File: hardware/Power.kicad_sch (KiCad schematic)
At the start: 8 parts, among them U201 TPS62172DSGR

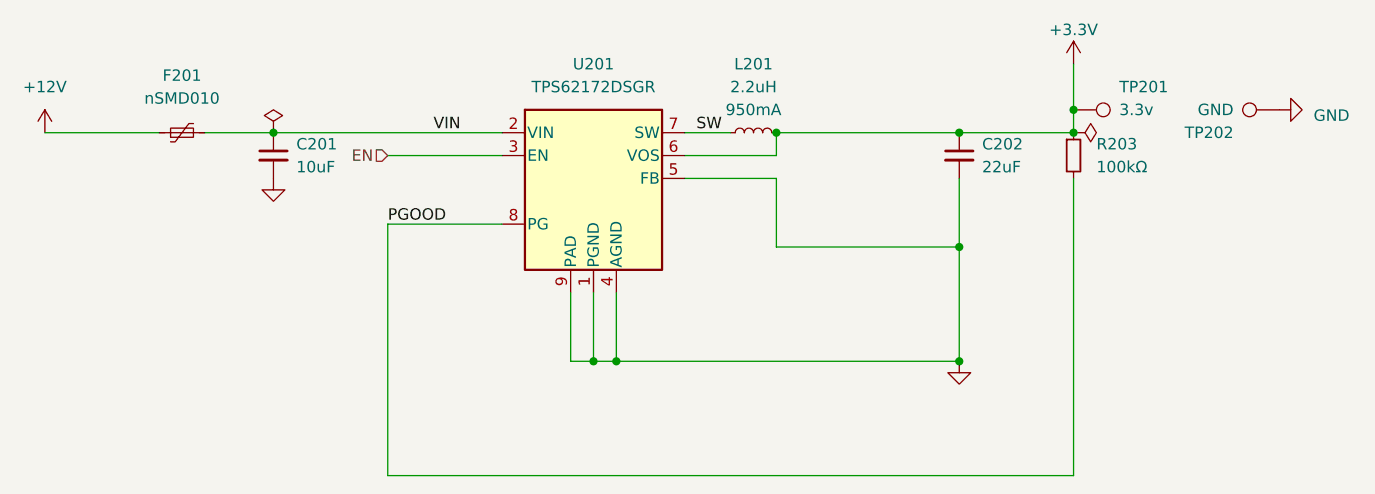
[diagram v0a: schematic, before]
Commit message: Almost ready for fab
Signed-off-by: Connor Rigby <connorr@hey.com>
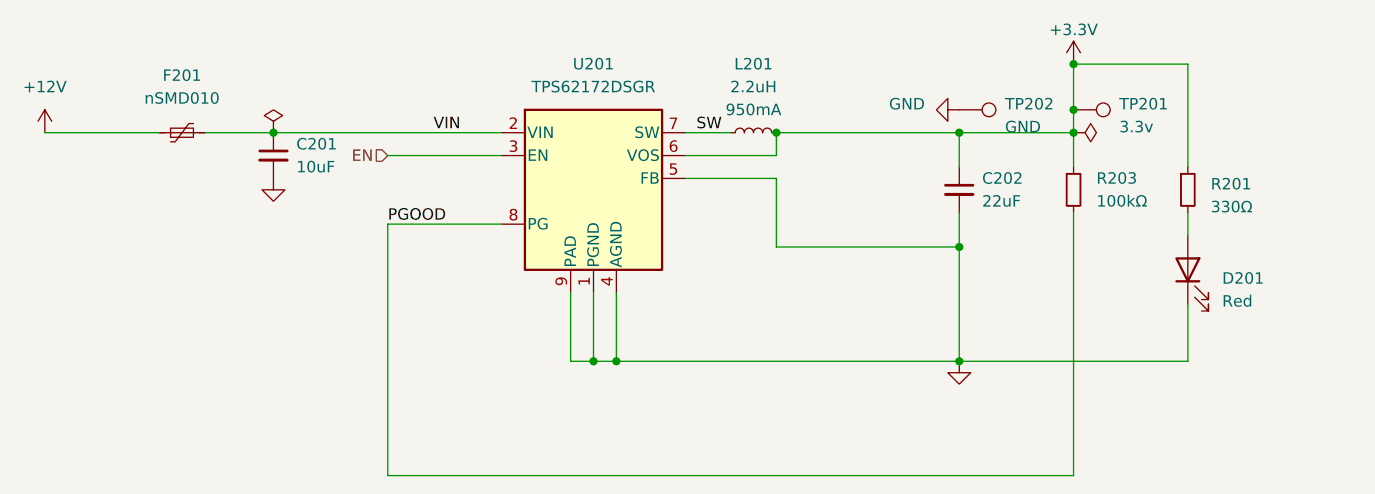
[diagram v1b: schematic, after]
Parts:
- added D201: LED_0603_RED, LED_SMD:LED_0603_1608Metric, symbol LCSC_LED:LED_0603_RED
- added R201: R_0603_330, Resistor_SMD:R_0603_1608Metric, symbol LCSC_Resistor:R_0603_330
- TP201, TP202: now left out of the parts list
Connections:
- net +3.3V: now also R201.1
- net GND: now also D201.1 (K)
- new net: D201.2 (A), R201.2
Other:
- moved on the sheet: C202, R203, TP202
